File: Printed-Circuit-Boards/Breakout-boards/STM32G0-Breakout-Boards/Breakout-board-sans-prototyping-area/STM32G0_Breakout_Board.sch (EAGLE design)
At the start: 13 parts, among them U1 STM32G0_SO8_T2

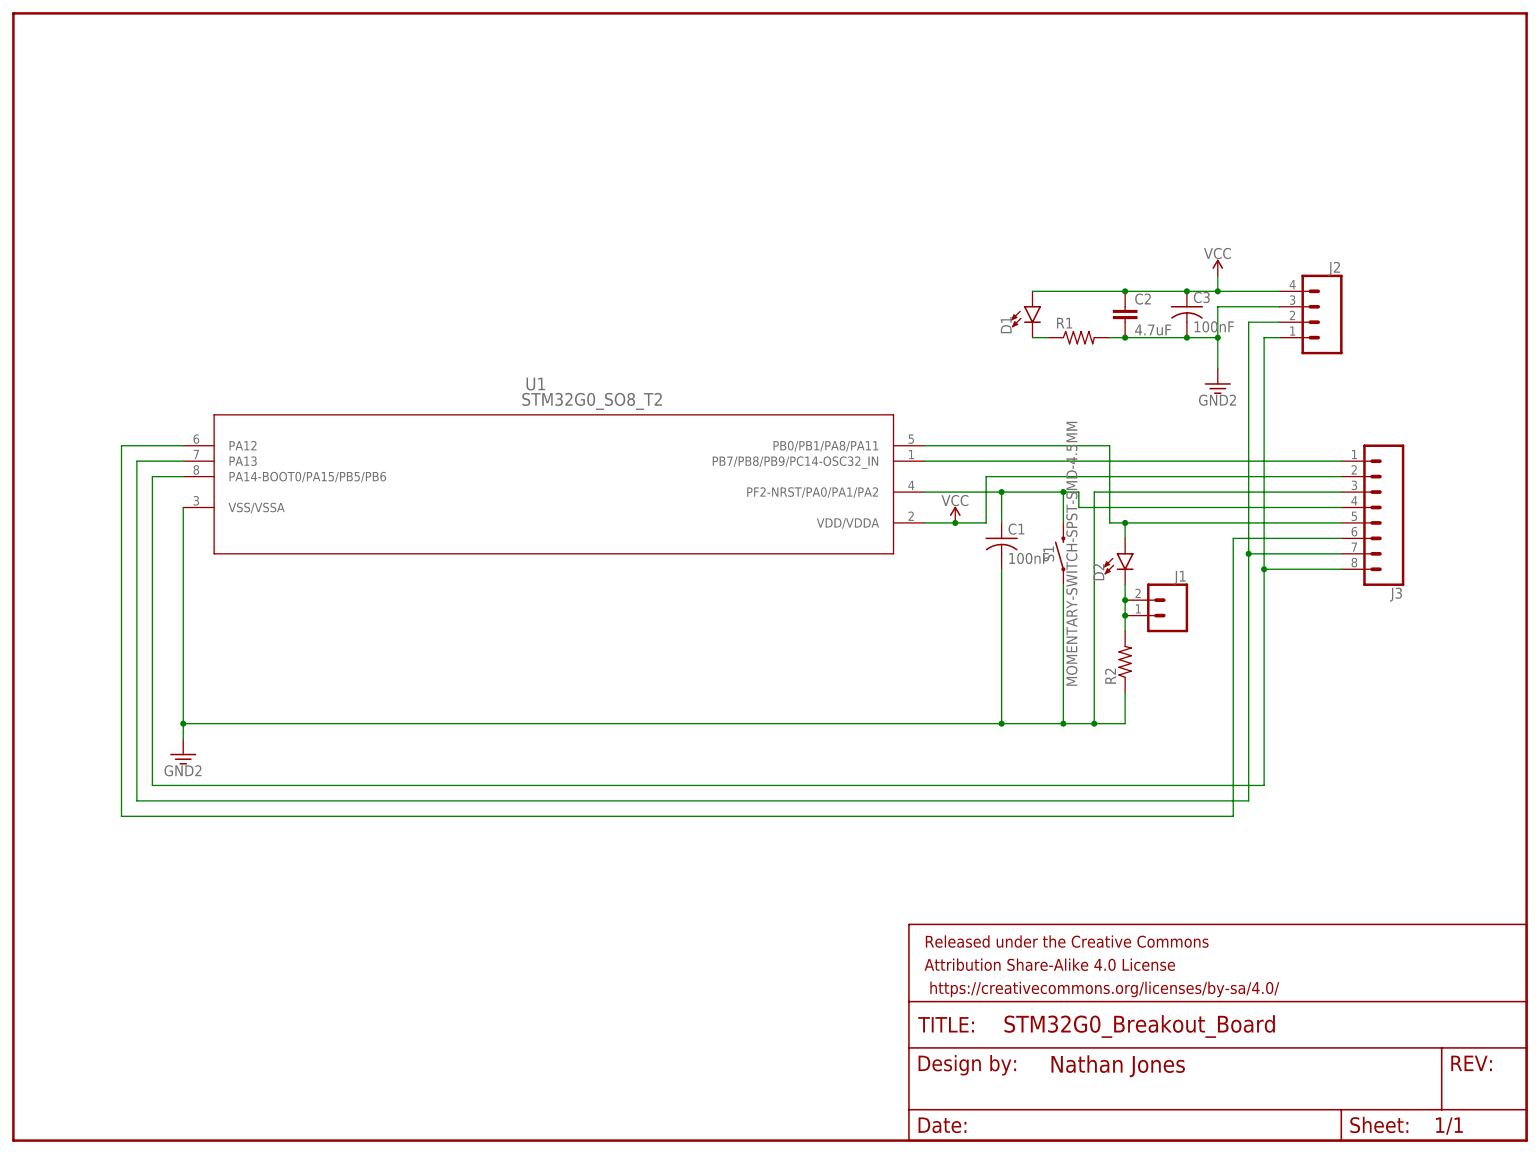
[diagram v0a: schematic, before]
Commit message: Updated PCB files.
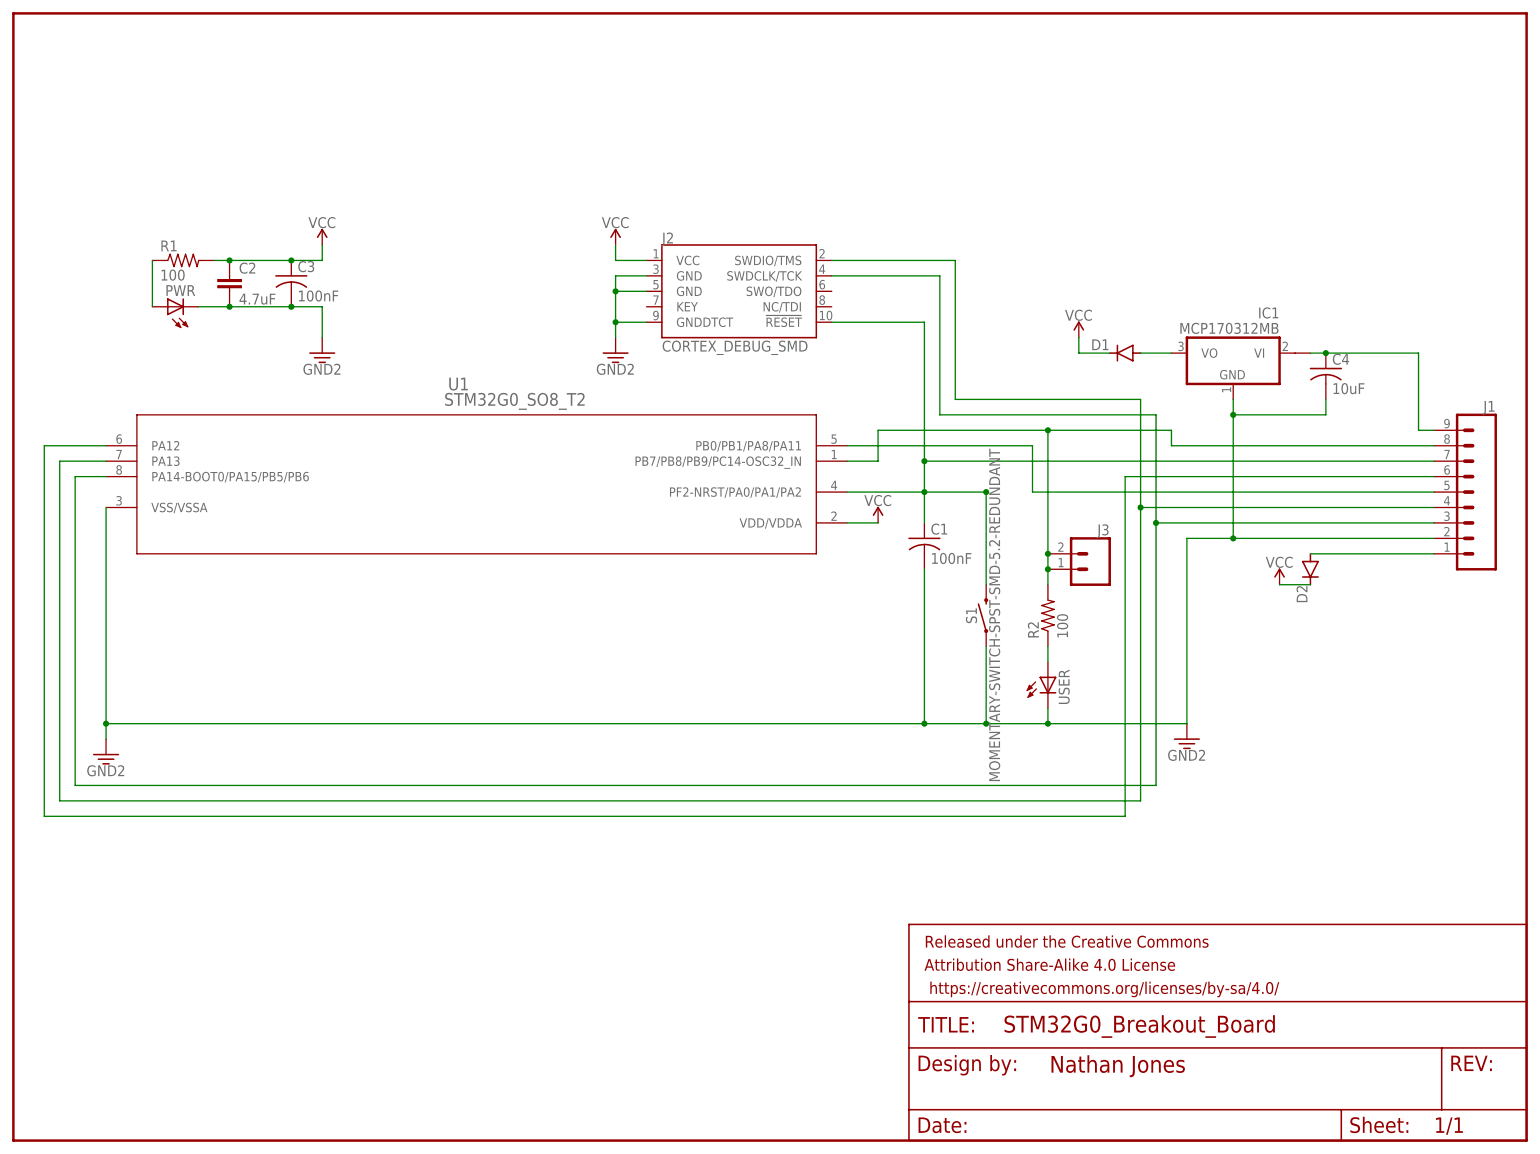
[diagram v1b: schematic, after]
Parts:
- added C4: 10uF, adafruit:C-USC1206
- added IC1: MCP170312MB, linear:MCP170312MB
- added PWR, USER: (no value), adafruit:LEDCHIP-LED0805
- D1, D2: device SparkFun-LED:LED1206 -> diode:DIODE-DO-214AC
- J1: device SparkFun-Connectors:CONN_02PTH3 -> SparkFun-Connectors:CONN_09LONGPADS
- J2: value (none) -> CORTEX_DEBUG_SMD; device SparkFun-Connectors:CONN_04LONGPADS -> SparkFun-Connectors:CORTEX_DEBUG_SMD
- J3: device SparkFun-Connectors:CONN_08LONGPADS -> SparkFun-Connectors:CONN_02PTH3
- R1, R2: value (none) -> 100
- S1: value MOMENTARY-SWITCH-SPST-SMD-4.5MM -> MOMENTARY-SWITCH-SPST-SMD-5.2-REDUNDANT; device SparkFun-Switches:MOMENTARY-SWITCH-SPST-SMD-4.5MM -> SparkFun-Switches:MOMENTARY-SWITCH-SPST-SMD-5.2-REDUNDANT
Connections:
- removed net N$11: D1.C, R1.1
- removed net PB7/PB8/PB9/PC14: J3.1, U1.PB7/PB8/PB9/PC14-OSC32_IN
- new net N$2: D2.A, J1.1
- new net N$3: C4.1, IC1.VI1, J1.9
- new net N$4: PWR.A, R1.1
- new net N$5: D1.A, IC1.VO
- new net PC14: J1.8, J3.1, J3.2, R2.2, U1.PB7/PB8/PB9/PC14-OSC32_IN
- net GND: now also C4.2, IC1.GND, J1.2, J2.GND@3, J2.GND@5, J2.GNDDTCT, PWR.C, USER.C; no longer J2.3, J3.3, R1.2, R2.1
- net N$1: now also R2.1, USER.A; no longer D2.C, J1.1, J1.2, R2.2
- net NRST/PA0/PA1/PA2: now also J1.7, J2.!RESET; no longer J3.4
- net PA12: now also J1.6; no longer J3.6
- net PB0/PB1/PA8/PA11: now also J1.5; no longer D2.A, J3.5
- net SWDCLK: now also J1.3, J2.SWDCLK/TCK; no longer J2.1, J3.8
- net SWDIO: now also J1.4, J2.SWDIO/TMS; no longer J2.2, J3.7
- net VCC: now also D1.C, D2.C, J2.VCC, R1.2; no longer D1.A, J2.4, J3.2
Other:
- moved on the sheet: C1, C2, C3, R1, R2, S1, U1
